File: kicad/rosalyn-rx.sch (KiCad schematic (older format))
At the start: 36 parts, among them J2 Serial1, J3 Serial2, J4 PWM, U1 STM32F303CCTx, U2 E22-EBYTE, U3 XC6206P330MR, U4 TXS0108EPW, U5 BMP280, U6 ICM-20602

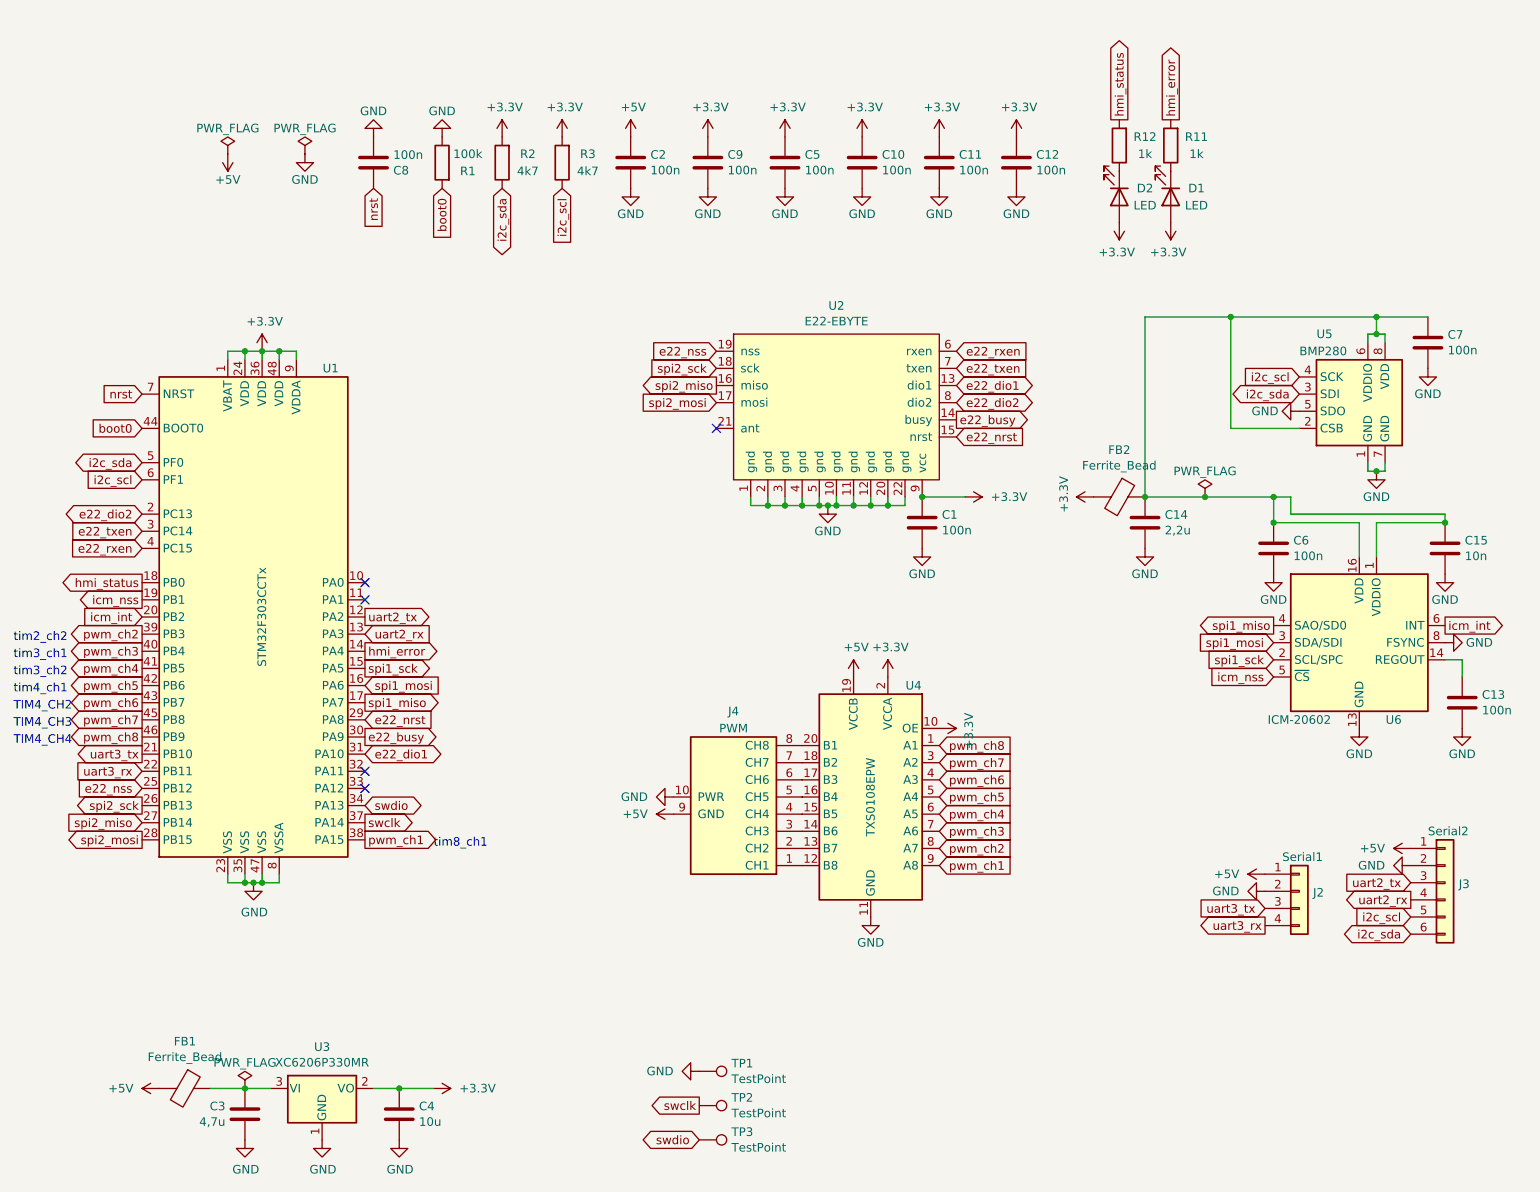
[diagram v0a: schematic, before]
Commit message: updated nvdata driver
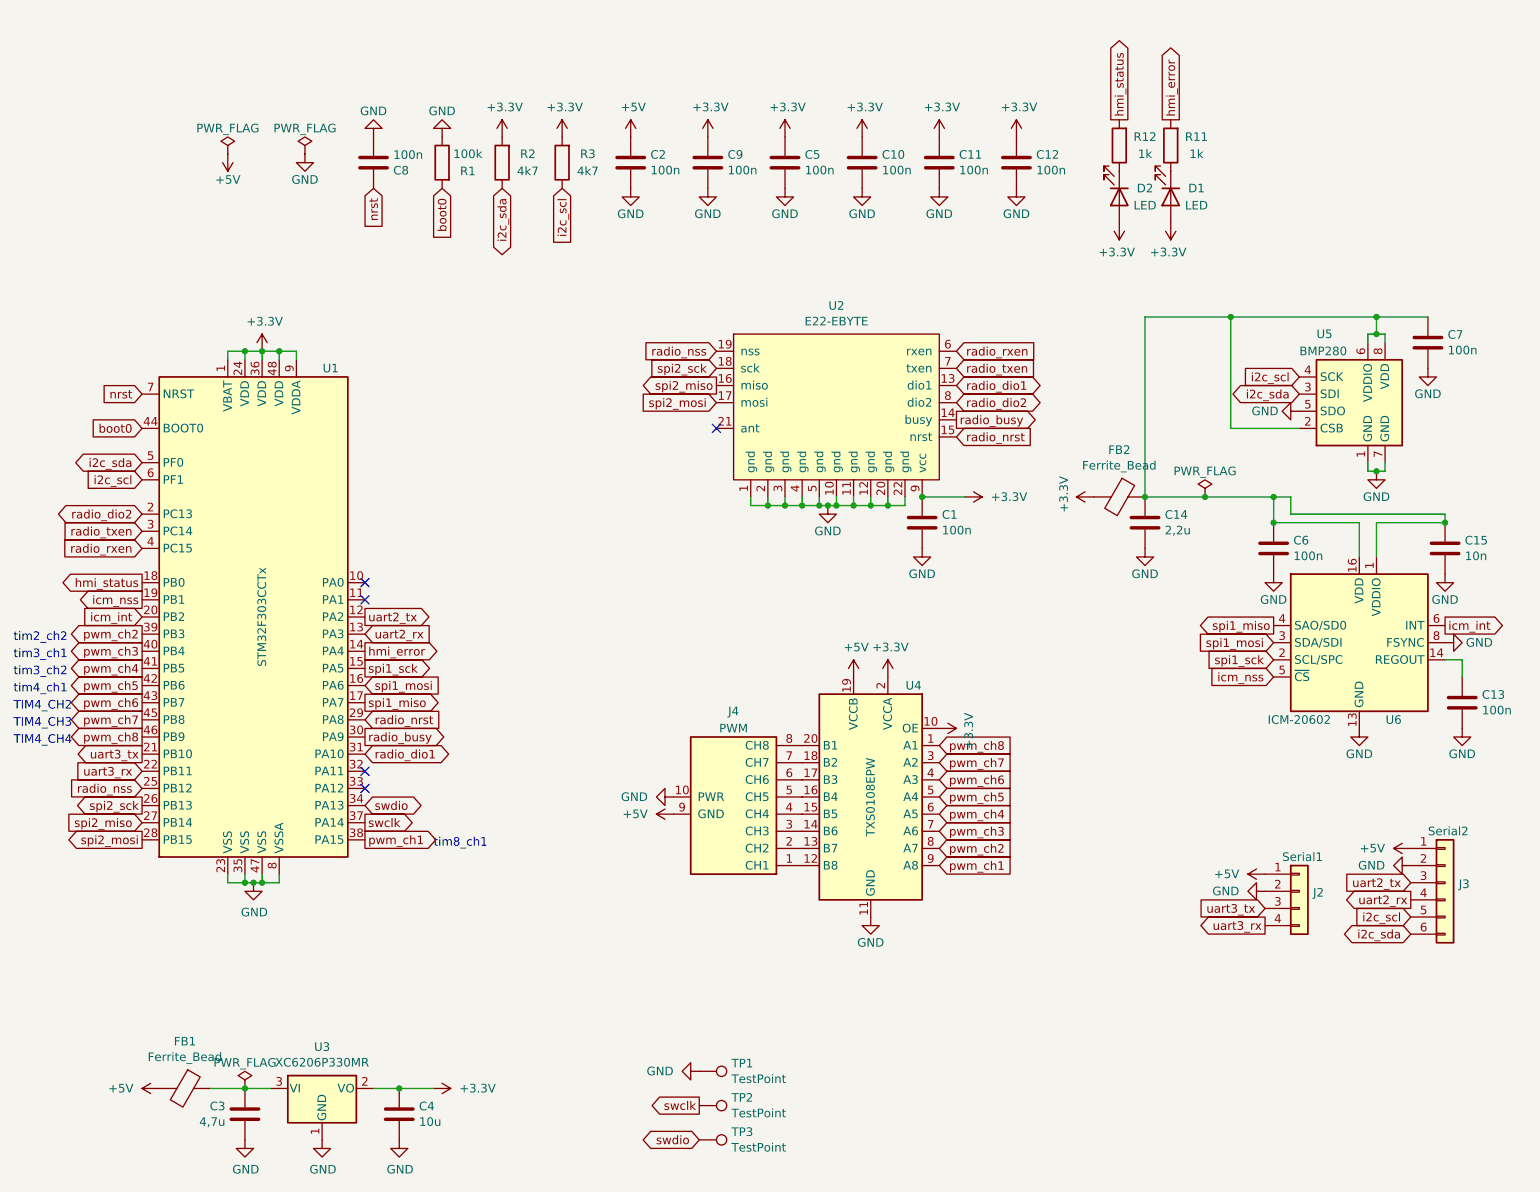
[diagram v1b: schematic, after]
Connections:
- net e22_busy renamed radio_busy
- net e22_dio1 renamed radio_dio1
- net e22_dio2 renamed radio_dio2
- net e22_nrst renamed radio_nrst
- net e22_nss renamed radio_nss
- net e22_rxen renamed radio_rxen
- net e22_txen renamed radio_txen
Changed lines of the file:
@@
 Sheet 1 1
 Title "RosalynRX"
-Date "2020-11-17"
+Date "2020-11-23"
 Rev "v1.0"
 Comp "www.2-0.dk"
@@
 NoConn ~ 6000 3100
 Text GLabel 6000 2650 0    50   Input ~ 0
-e22_nss
+radio_nss
 Text GLabel 6000 2750 0    50   Input ~ 0
 spi2_sck
@@
 spi2_mosi
 Text GLabel 7400 2650 2    50   Input ~ 0
-e22_rxen
+radio_rxen
 Text GLabel 7400 2750 2    50   Input ~ 0
-e22_txen
+radio_txen
 Text GLabel 7400 2850 2    50   BiDi ~ 0
-e22_dio1
+radio_dio1
 Text GLabel 7400 2950 2    50   BiDi ~ 0
-e22_dio2
+radio_dio2
 Text GLabel 7400 3050 2    50   Output ~ 0
-e22_busy
+radio_busy
 Text GLabel 7400 3150 2    50   Input ~ 0
-e22_nrst
+radio_nrst
 Text GLabel 3950 4500 2    50   Output ~ 0
 spi1_sck
@@
 spi2_mosi
 Text GLabel 2650 5200 0    50   Input ~ 0
-e22_nss
+radio_nss
 Text GLabel 3950 4800 2    50   Input ~ 0
-e22_nrst
+radio_nrst
 Text GLabel 3950 4900 2    50   Output ~ 0
-e22_busy
+radio_busy
 Text GLabel 3950 5000 2    50   BiDi ~ 0
-e22_dio1
+radio_dio1
 Text GLabel 2650 3600 0    50   BiDi ~ 0
-e22_dio2
+radio_dio2
 Text GLabel 2650 3700 0    50   Input ~ 0
-e22_txen
+radio_txen
 Text GLabel 2650 3800 0    50   Input ~ 0
-e22_rxen
+radio_rxen
 Text GLabel 9250 4550 0    50   Input ~ 0
 icm_nss
